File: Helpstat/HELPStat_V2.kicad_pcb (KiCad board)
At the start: 2 copper layers, 48 parts, among them J1 10118192-0001LF, J2 LIPO1, J3 M20-9990246, J4 M20-9990246, J5 M20-9990246, J6 M50-3530442, J7 M50-3530442, J8 M50-3530442, U1 ESP32-DEVKITC-32D, U2 MCP73831T-2ACI/OT, U3 AP2112K-3.3TRG1, U4 AD5941BCPZ-RL7

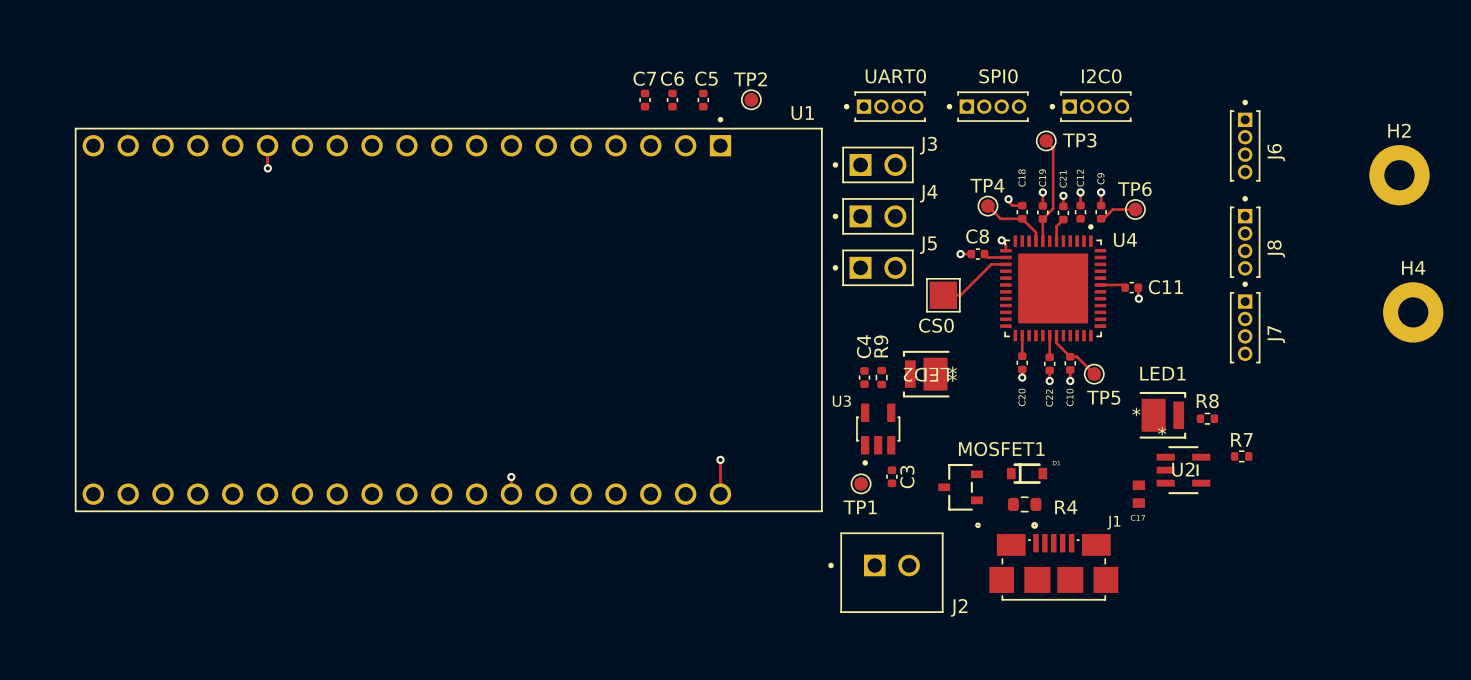
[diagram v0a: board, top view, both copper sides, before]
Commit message: more pcb changes
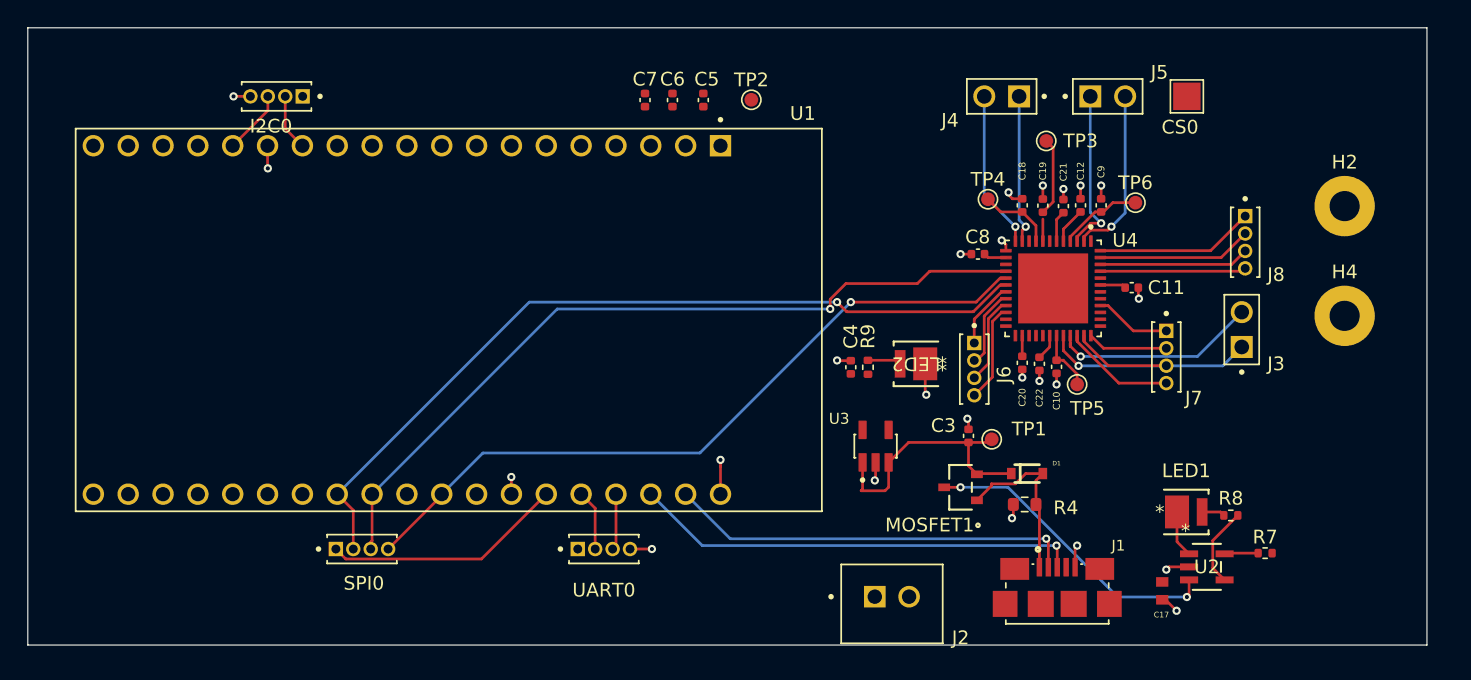
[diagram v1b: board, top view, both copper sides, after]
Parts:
- moved I2C0 59.7 mm to (53.6, 94.5), turned to 180 degrees
- moved SPI0 56.2 mm to (59.9, 127.5)
- moved UART0 38.4 mm to (77.5, 127.5)
- moved J3 29.1 mm to (124.0, 111.5), turned to 90 degrees
- moved J6 25.6 mm to (104.5, 114.4)
- moved CS0 22.9 mm to (120.0, 94.5)
- moved J5 20.9 mm to (114.2, 94.5)
- moved J4 12.6 mm to (106.5, 94.5), turned to 180 degrees
- moved TP1 10.1 mm to (105.8, 119.5), turned to 180 degrees
- moved C17 7.25 mm to (118.2, 130.5)
- moved U2 7.25 mm to (121.5, 128.8)
- moved LED1 7.25 mm to (120.0, 124.8)
- moved R7 7.25 mm to (125.7, 127.8)
- moved R8 7.25 mm to (123.2, 125.0)
- moved C3 6.33 mm to (104.1, 119.2), turned to 90 degrees
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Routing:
- net /MISO: track 0.00 -> 60.1 mm, vias 0 -> 1
- net /SCLK: track 0.00 -> 57.4 mm, vias 0 -> 1
- net /MOSI: track 0.00 -> 53.3 mm, vias 0 -> 1
- net /USB_P: track 0.00 -> 32.7 mm, vias 0 -> 1
- net /USB_N: track 0.00 -> 29.8 mm, vias 0 -> 1
- net VLIPO: track 0.00 -> 22.3 mm, vias 0 -> 2
- net Net-(MOSFET1-S): track 0.00 -> 19.3 mm
- net VUSB: track 0.00 -> 18.6 mm
- net /CS.SPI: track 0.00 -> 17.6 mm
- net /RCAL1: track 0.00 -> 15.2 mm, vias 0 -> 1
- net /RCAL0: track 0.00 -> 15.1 mm, vias 0 -> 1
- net GND: track 15.1 -> 29.1 mm, vias 14 -> 24
- net /RC0.1: track 0.00 -> 12.5 mm, vias 0 -> 1
- net /RC0.0: track 0.00 -> 12.1 mm, vias 0 -> 1
- net /RE: track 0.00 -> 11.6 mm
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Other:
- board outline added: 102 x 45 mm
